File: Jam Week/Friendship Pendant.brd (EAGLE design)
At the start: 43.2 x 43.2 mm, 40 parts, among them IC1 LM556D, IC2 LM556D, IC3 74AHC1G32DCK, U1 3039

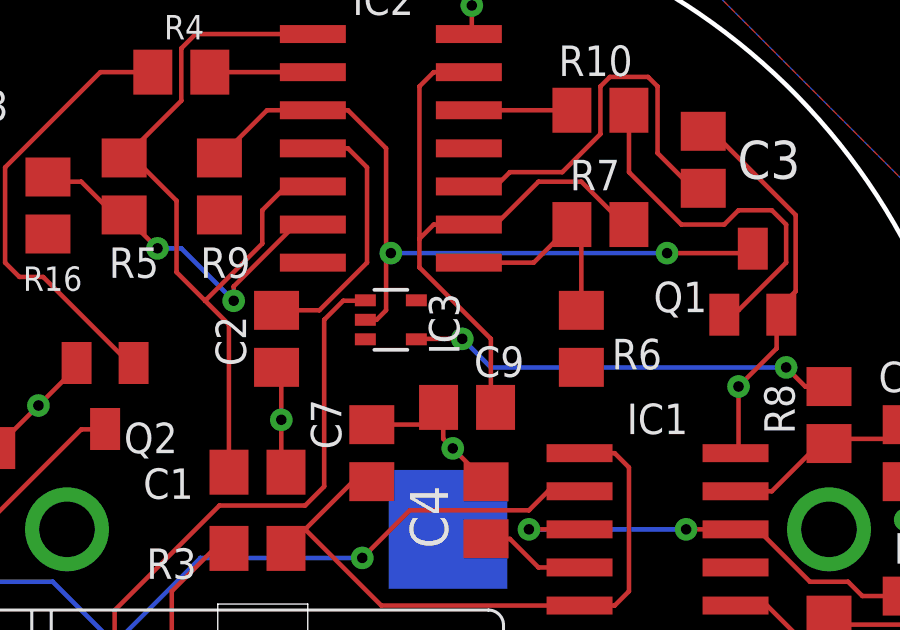
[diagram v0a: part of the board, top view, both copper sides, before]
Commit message: final day
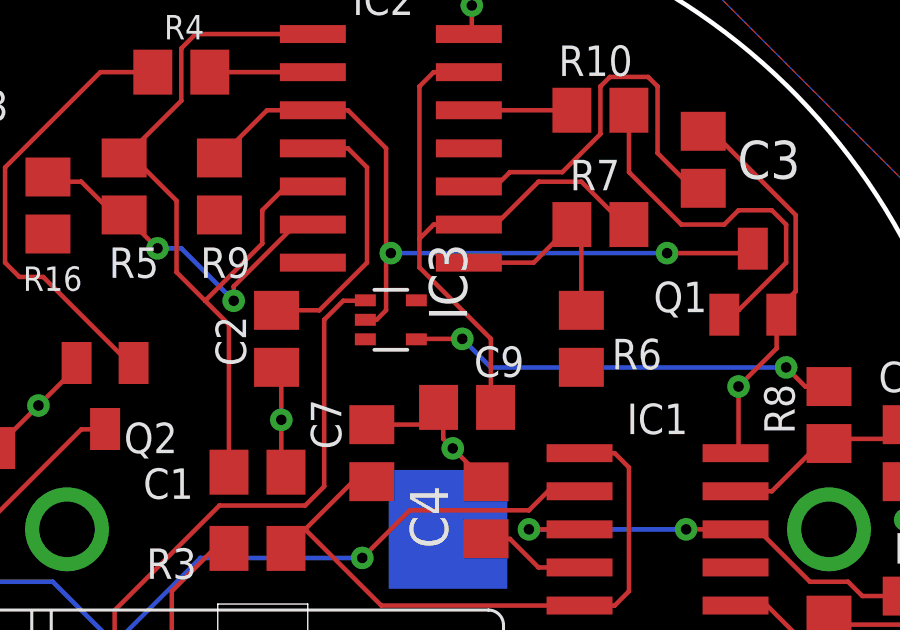
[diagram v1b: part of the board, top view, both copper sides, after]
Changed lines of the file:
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@@
 <attribute name="MOUSER#" value="595-SN74AUP1G32DCKR" x="18.415" y="28.575" size="1.778" layer="27" rot="R270" display="off"/>
 <attribute name="MPN" value="SN74AUP1G32DCKR" x="18.415" y="28.575" size="1.778" layer="27" rot="R270" display="off"/>
-<attribute name="NAME" x="50.165" y="54.864" size="1.016" layer="25" rot="R270"/>
+<attribute name="NAME" x="50.165" y="56.515" size="1.27" layer="25" rot="R270"/>
 <attribute name="VALUE" x="46.355" y="56.515" size="1.27" layer="27" rot="R270"/>
 </element>
@@
 <contactref element="R6" pad="2"/>
 <contactref element="S1" pad="3"/>
-<wire x1="55.245" y1="52.39" x2="60.385" y2="45.72" width="0" layer="19" extent="1-1"/>
-<wire x1="49.745" y1="54.625" x2="55.245" y2="52.39" width="0" layer="19" extent="1-1"/>
-<wire x1="46.295" y1="55.88" x2="49.745" y2="54.625" width="0" layer="19" extent="1-1"/>
-<wire x1="43.18" y1="57.47" x2="46.295" y2="55.88" width="0" layer="19" extent="1-1"/>
-<wire x1="37.465" y1="56.835" x2="43.18" y2="57.47" width="0" layer="19" extent="1-1"/>
-<wire x1="31.115" y1="52.385" x2="37.465" y2="56.835" width="0" layer="19" extent="1-1"/>
-<wire x1="34.925" y1="39.37" x2="31.115" y2="52.385" width="0" layer="19" extent="1-1"/>
-<wire x1="31.115" y1="35.245" x2="34.925" y2="39.37" width="0" layer="19" extent="1-1"/>
-<wire x1="37.15" y1="29.845" x2="31.115" y2="35.245" width="0" layer="19" extent="1-1"/>
-<wire x1="41.595" y1="29.675" x2="37.15" y2="29.845" width="0" layer="19" extent="1-1"/>
-<wire x1="21.336" y1="32.513" x2="31.115" y2="35.245" width="0" layer="19" extent="1-1"/>
+<wire x1="31.115" y1="35.245" x2="21.336" y2="32.513" width="0" layer="19" extent="1-1"/>
 </signal>
 <signal name="N$1">
